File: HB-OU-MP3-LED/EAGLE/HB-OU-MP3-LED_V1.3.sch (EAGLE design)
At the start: 22 parts, among them Q1 BC327, X1 MSTBA2, X3 MSTBA3

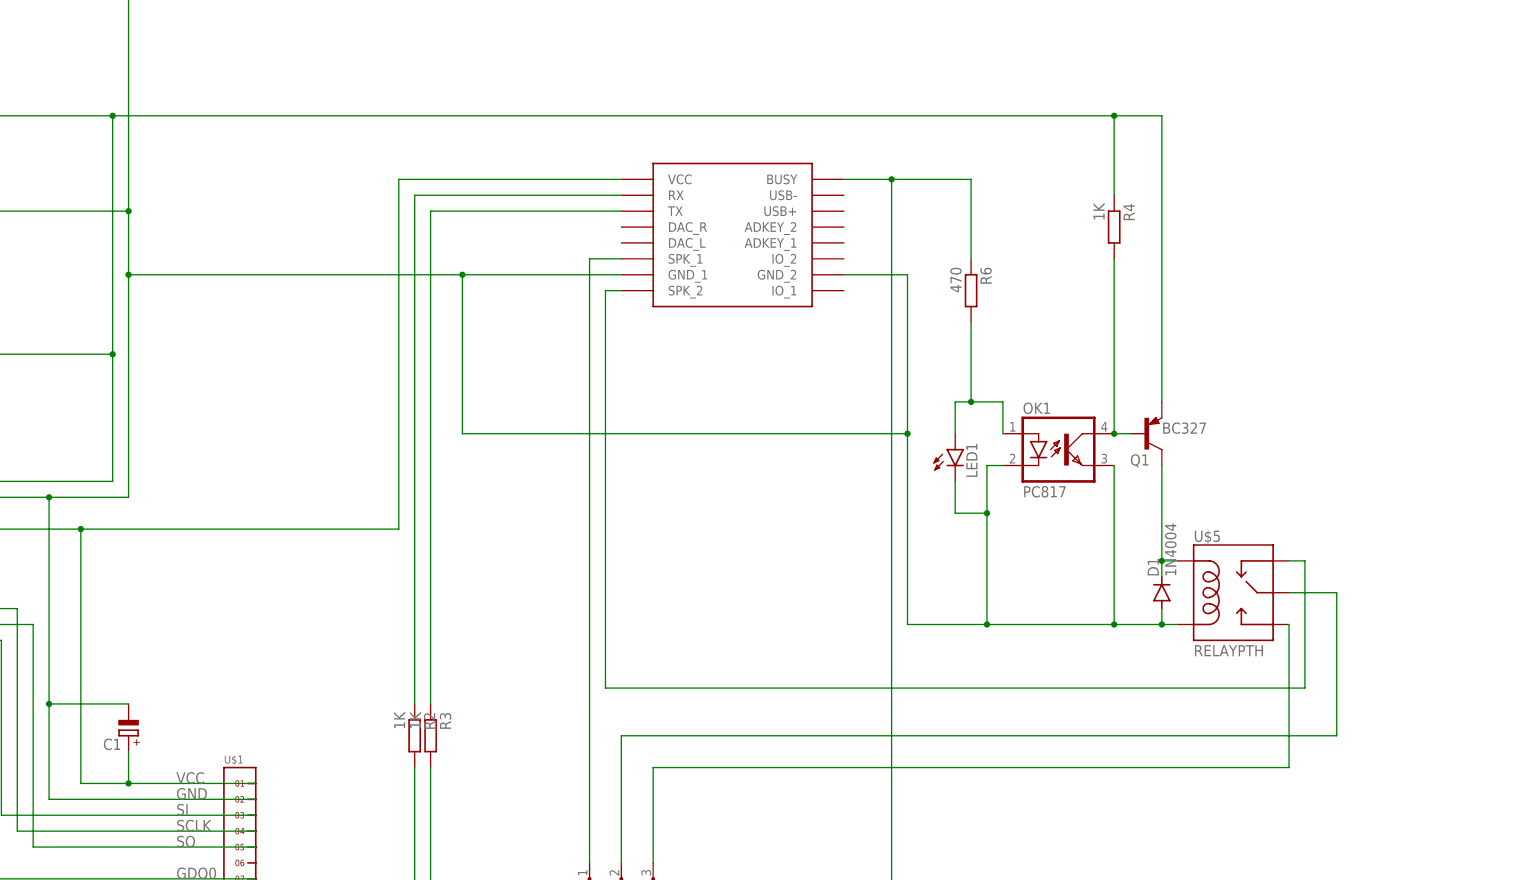
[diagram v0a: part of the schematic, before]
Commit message: Update HB-OU-MP3-LED_V1.3.sch
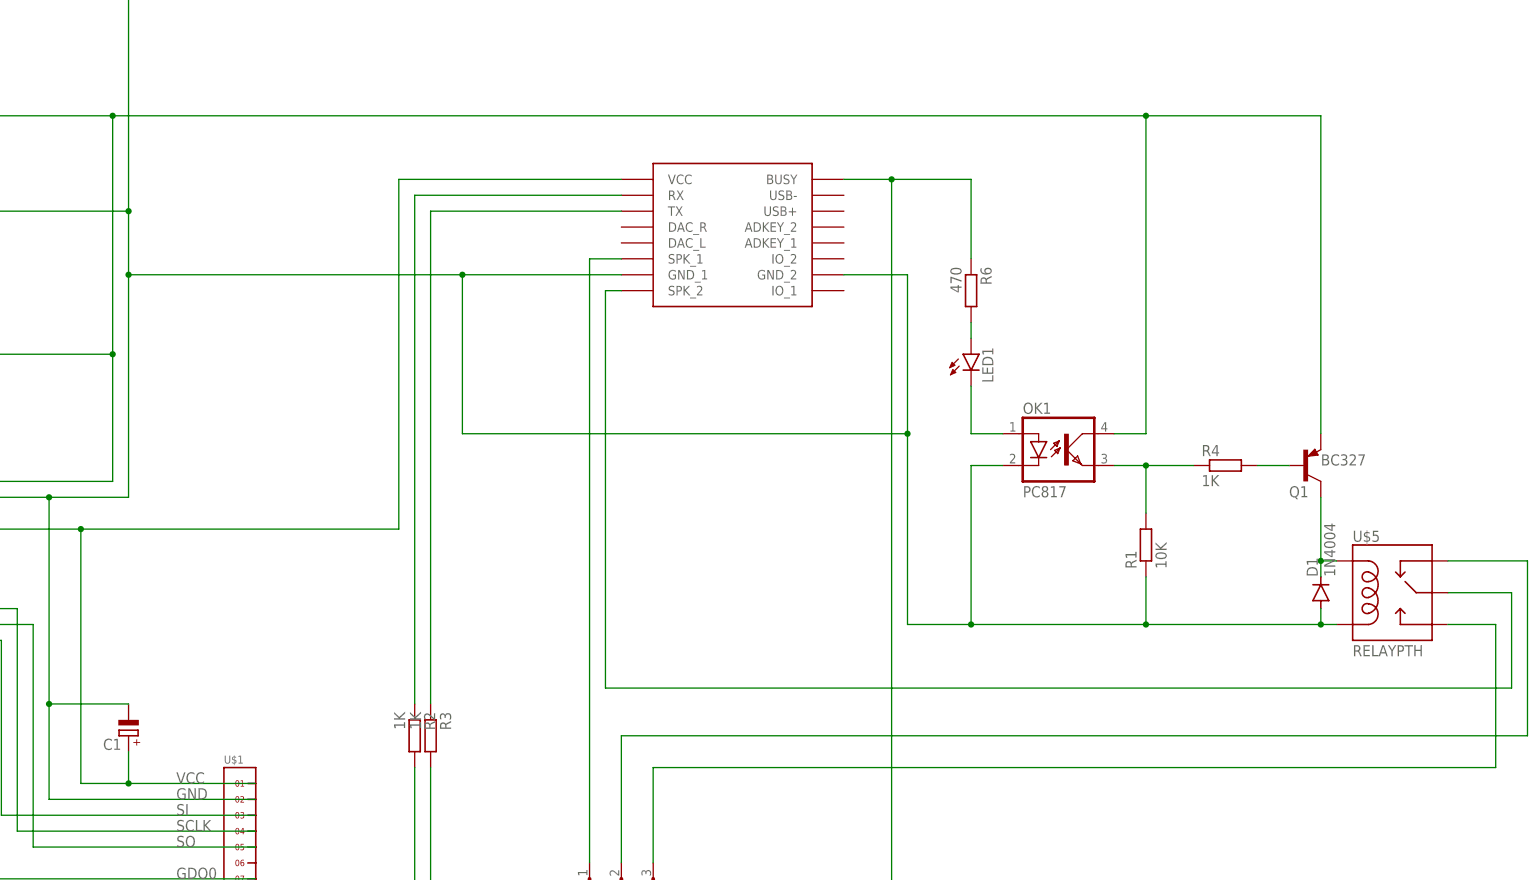
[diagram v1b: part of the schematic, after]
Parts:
- added R1: 10K, resistor:R-EU_0309/10
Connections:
- new net N$21: LED1.C, OK1.A
- new net N$22: Q1.B, R4.2
- net GND: now also R1.1; no longer LED1.C, OK1.EMIT
- net N$13: now also U$5.SWCLOSE; no longer U$5.SWCOMMON
- net N$16: now also OK1.EMIT, R1.2, R4.1; no longer OK1.COL, Q1.B, R4.2
- net N$7: now also U$5.SWCOMMON; no longer U$5.SWCLOSE
- net N$8: no longer OK1.A
- net RAW: now also OK1.COL; no longer R4.1
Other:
- moved on the sheet: D1, LED1, Q1, R4, U$5
